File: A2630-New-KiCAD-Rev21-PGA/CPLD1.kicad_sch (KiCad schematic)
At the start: 19 parts, among them CN600 CPLD0, CN601 CPLD1, CN602 CPLD2, J600 IDE DISABLE, U600 XC9572XL-VQ64, U601 XC95144XL-TQ144, U602 XC95144XL-TQ144

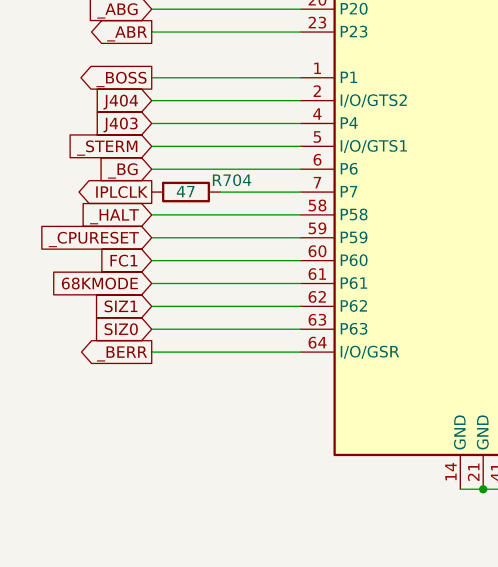
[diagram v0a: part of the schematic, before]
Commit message: Add files via upload
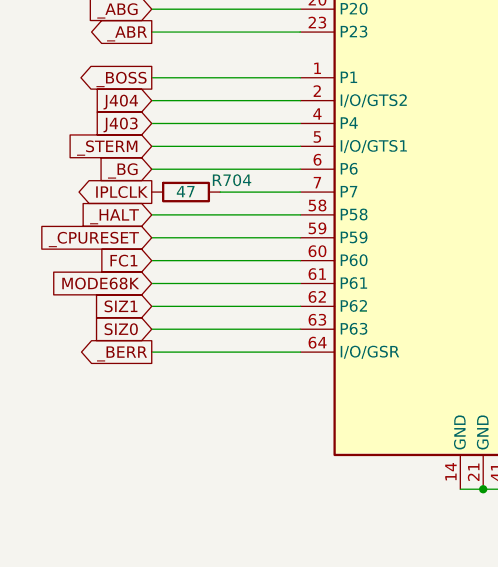
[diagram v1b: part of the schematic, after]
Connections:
- net 68KMODE is gone; now on net MODE68K: U600.61 (P61)
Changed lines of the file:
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@@
     )
   )
-  (global_label "68KMODE" (shape input) (at 37.465 155.575 180) (fields_autoplaced)
+  (global_label "MODE68K" (shape input) (at 37.465 155.575 180) (fields_autoplaced)
     (effects (font (size 1.27 1.27)) (justify right))
     (property "Intersheet References" "${INTERSHEET_REFS}" (id 0) (at 26.2508 155.4956 0)
